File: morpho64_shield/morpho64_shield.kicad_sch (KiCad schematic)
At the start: 7 parts, among them J1 CN7, J2 CN10, SW1 SW_DIP_x08

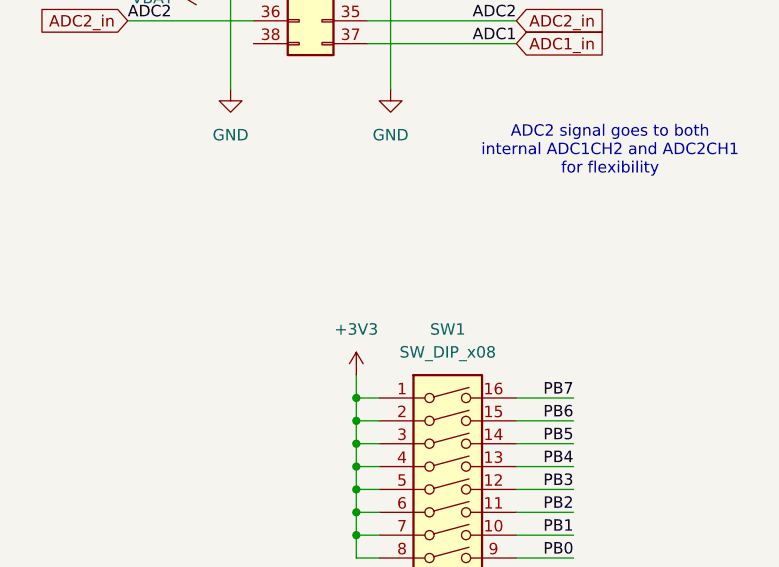
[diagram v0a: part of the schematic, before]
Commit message: First PCB order
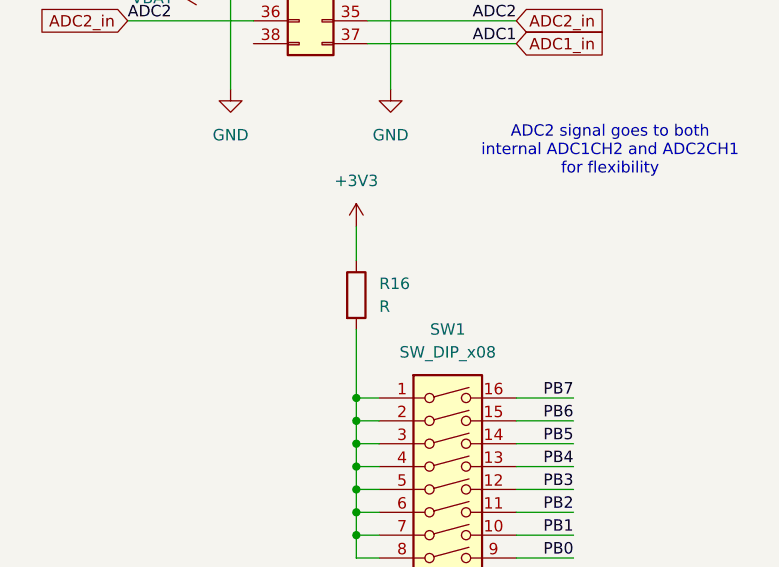
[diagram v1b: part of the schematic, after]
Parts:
- added R16: R, Resistor_SMD:R_0603_1608Metric, symbol Device:R
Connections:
- net +3V3: now also R16.1; no longer SW1.1, SW1.2, SW1.3, SW1.4, SW1.5, SW1.6, SW1.7, SW1.8
- new net: R16.2, SW1.1, SW1.2, SW1.3, SW1.4, SW1.5, SW1.6, SW1.7, SW1.8
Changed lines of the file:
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@@
 	(wire
 		(pts
+			(xy 55.88 140.97) (xy 55.88 148.59)
+		)
+		(stroke
+			(width 0)
+			(type default)
+		)
+	)
+	(wire
+		(pts
 			(xy 57.15 101.6) (xy 73.66 101.6)
 		)
@@
 	(wire
 		(pts
-			(xy 55.88 146.05) (xy 55.88 148.59)
+			(xy 55.88 129.54) (xy 55.88 133.35)
 		)
 		(stroke
@@
 	(symbol
 		(lib_id "power:+3V3")
-		(at 55.88 146.05 0)
+		(at 55.88 129.54 0)
 		(unit 1)
 		(body_style 1)
@@
 		(fields_autoplaced yes)
 		(property "Reference" "#PWR06"
-			(at 55.88 149.86 0)
+			(at 55.88 133.35 0)
 			(hide yes)
 			(show_name no)
@@
 		)
 		(property "Value" "+3V3"
-			(at 55.88 140.97 0)
+			(at 55.88 124.46 0)
 			(show_name no)
 			(do_not_autoplace no)
@@
 		)
 		(property "Footprint" ""
-			(at 55.88 146.05 0)
+			(at 55.88 129.54 0)
 			(hide yes)
 			(show_name no)
@@
 		)
 		(property "Datasheet" ""
-			(at 55.88 146.05 0)
+			(at 55.88 129.54 0)
 			(hide yes)
 			(show_name no)
@@
 		)
 		(property "Description" "Power symbol creates a global label with name \"+3V3\""
-			(at 55.88 146.05 0)
+			(at 55.88 129.54 0)
 			(hide yes)
 			(show_name no)
@@
 					(unit 1)
 				)
+			)
+		)
+	)
+	(symbol
+		(lib_id "Device:R")
+		(at 55.88 137.16 0)
+		(unit 1)
+		(body_style 1)
+		(exclude_from_sim no)
+		(in_bom yes)
+		(on_board yes)
+		(in_pos_files yes)
+		(dnp no)
+		(fields_autoplaced yes)
+		(property "Reference" "R16"
+			(at 58.42 135.8899 0)
+			(show_name no)
+			(do_not_autoplace no)
+			(effects
+				(font
+					(size 1.27 1.27)
+				)
+				(justify left)
+			)
+		)
+		(property "Value" "R"
+			(at 58.42 138.4299 0)
+			(show_name no)
+			(do_not_autoplace no)
+			(effects
+				(font
+					(size 1.27 1.27)
+				)
+				(justify left)
+			)
+		)
+		(property "Footprint" "Resistor_SMD:R_0603_1608Metric"
+			(at 54.102 137.16 90)
+			(hide yes)
+			(show_name no)
+			(do_not_autoplace no)
+			(effects
+				(font
+					(size 1.27 1.27)
+				)
+			)
+		)
+		(property "Datasheet" ""
+			(at 55.88 137.16 0)
+			(hide yes)
+			(show_name no)
+			(do_not_autoplace no)
+			(effects
+				(font
+					(size 1.27 1.27)
+				)
+			)
+		)
+		(property "Description" "Resistor"
+			(at 55.88 137.16 0)
+			(hide yes)
+			(show_name no)
+			(do_not_autoplace no)
+			(effects
+				(font
+					(size 1.27 1.27)
+				)
+			)
+		)
+		(pin "2"
+		)
+		(pin "1"
+		)
+		(instances
+			(project "morpho64_shield"
+				(path "/9278c48a-e3d9-46fc-9342-1a833157c1d8"
+					(reference "R16")
+					(unit 1)
+				)
